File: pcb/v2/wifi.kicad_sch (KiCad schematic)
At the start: 19 parts, among them U10 AIC8800, U14 TXS0102DCU, U16 TXS0102DCU

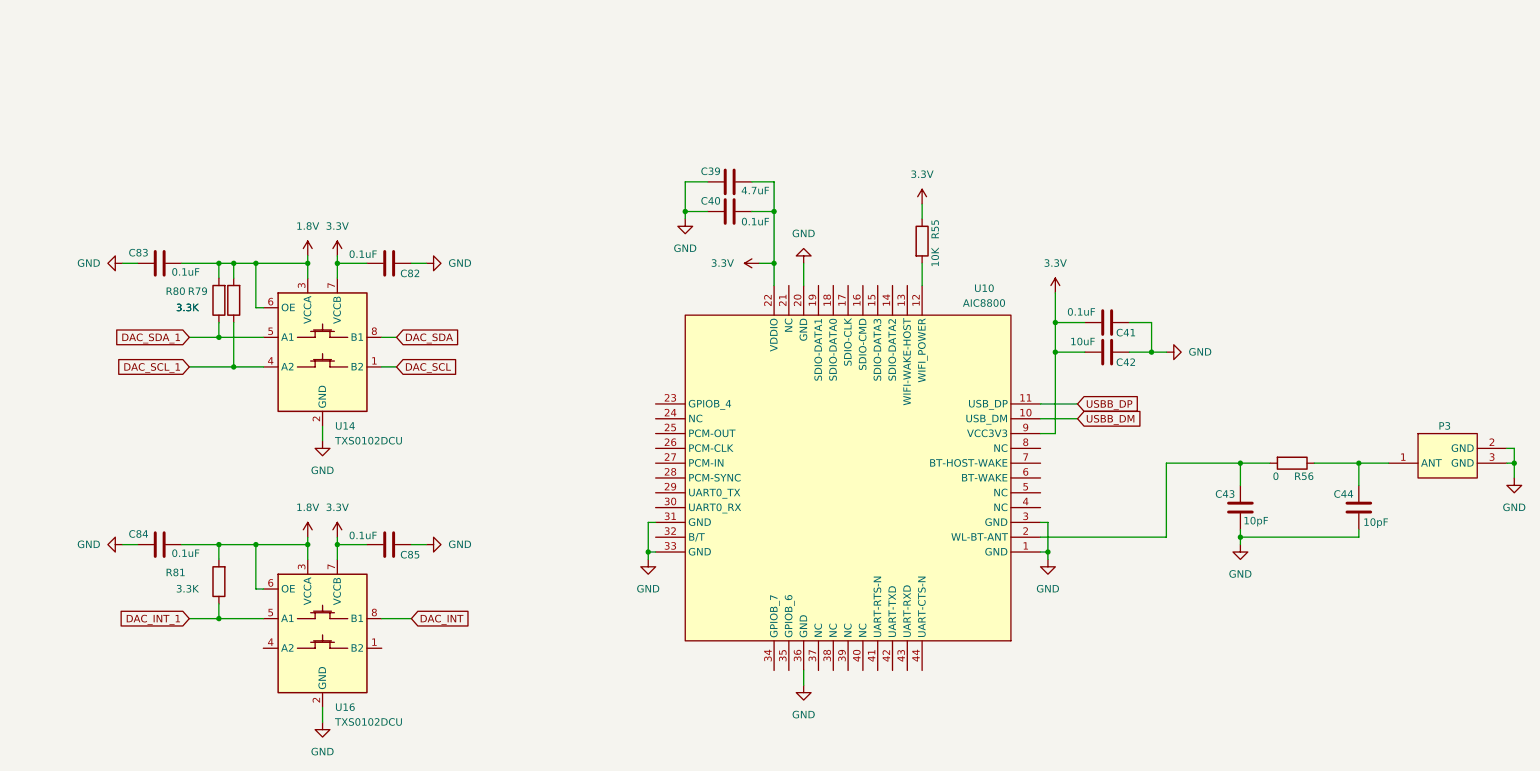
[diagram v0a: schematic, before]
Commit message: up
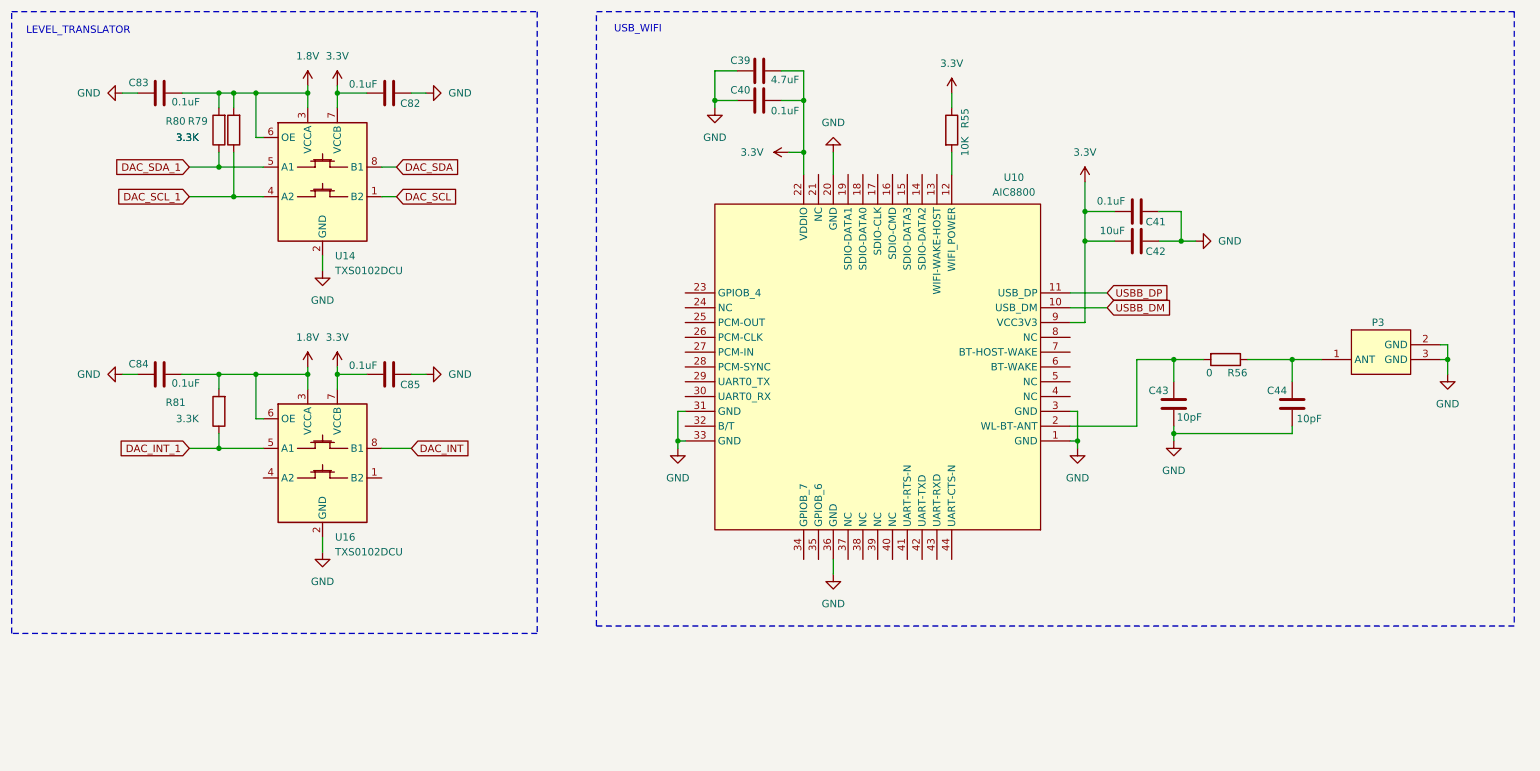
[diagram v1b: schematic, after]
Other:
- note added: "LEVEL_TRANSLATOR"
- note added: "USB_WIFI"
- moved on the sheet: C39, C40, C41, C42, C43, C44, C82, C83, C84, C85, P3, R55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
